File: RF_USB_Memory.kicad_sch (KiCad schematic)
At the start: 9 parts, among them J3 USB_B_Micro, U1 USBLC6-2SC6, U5 W25Q128JVSQ_SOIC208-mil

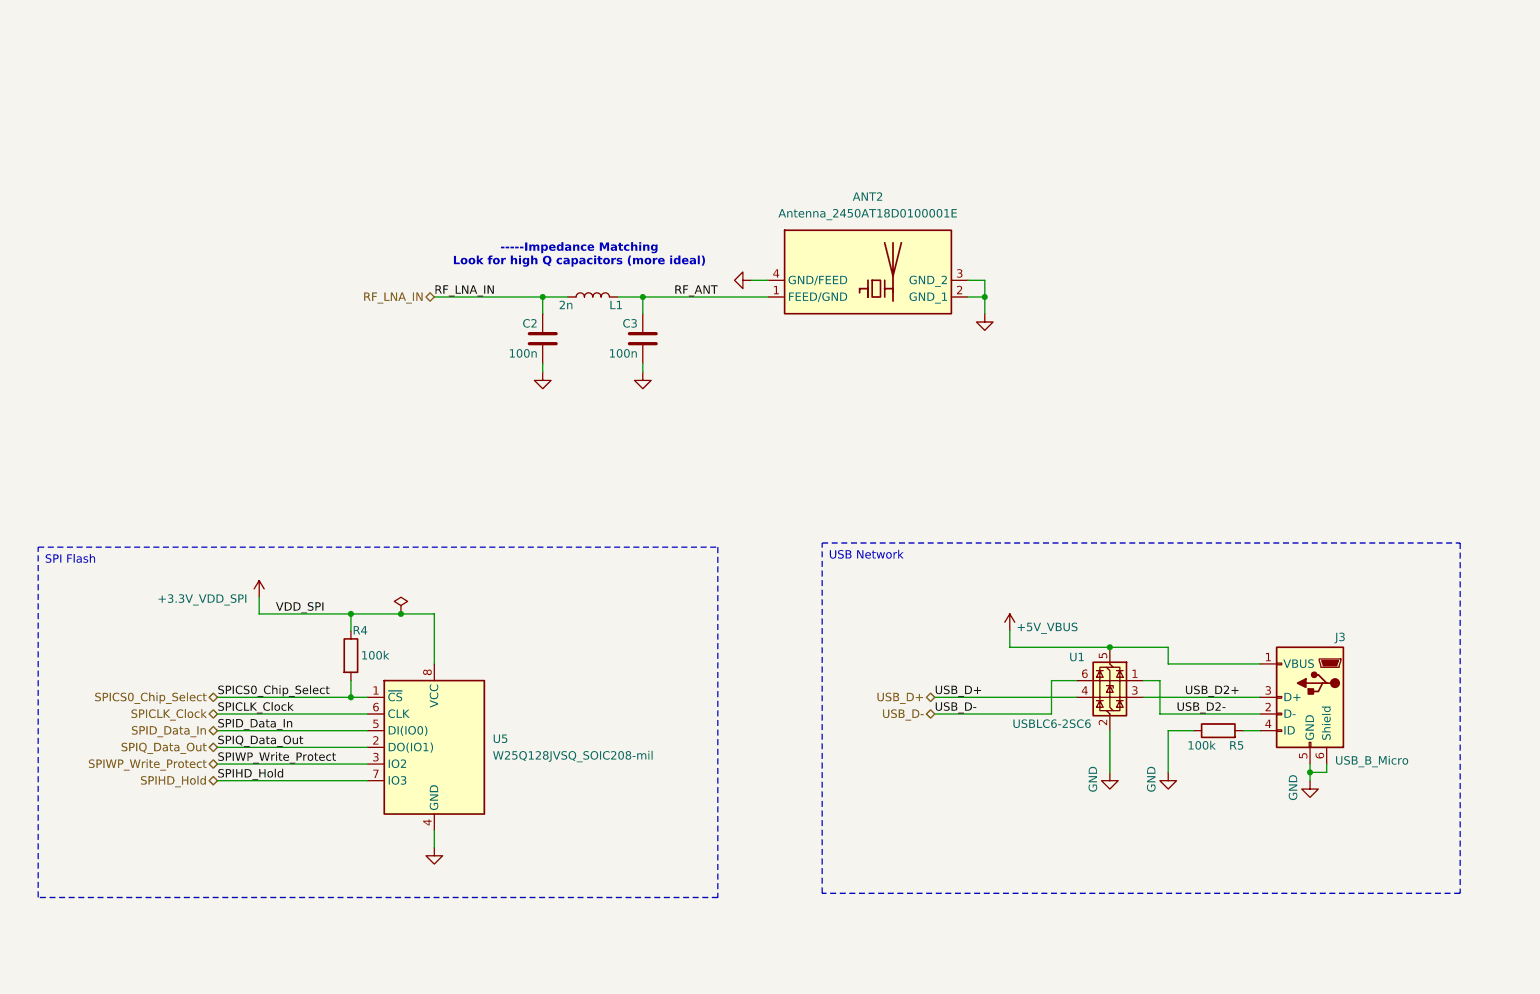
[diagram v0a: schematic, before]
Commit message: Update
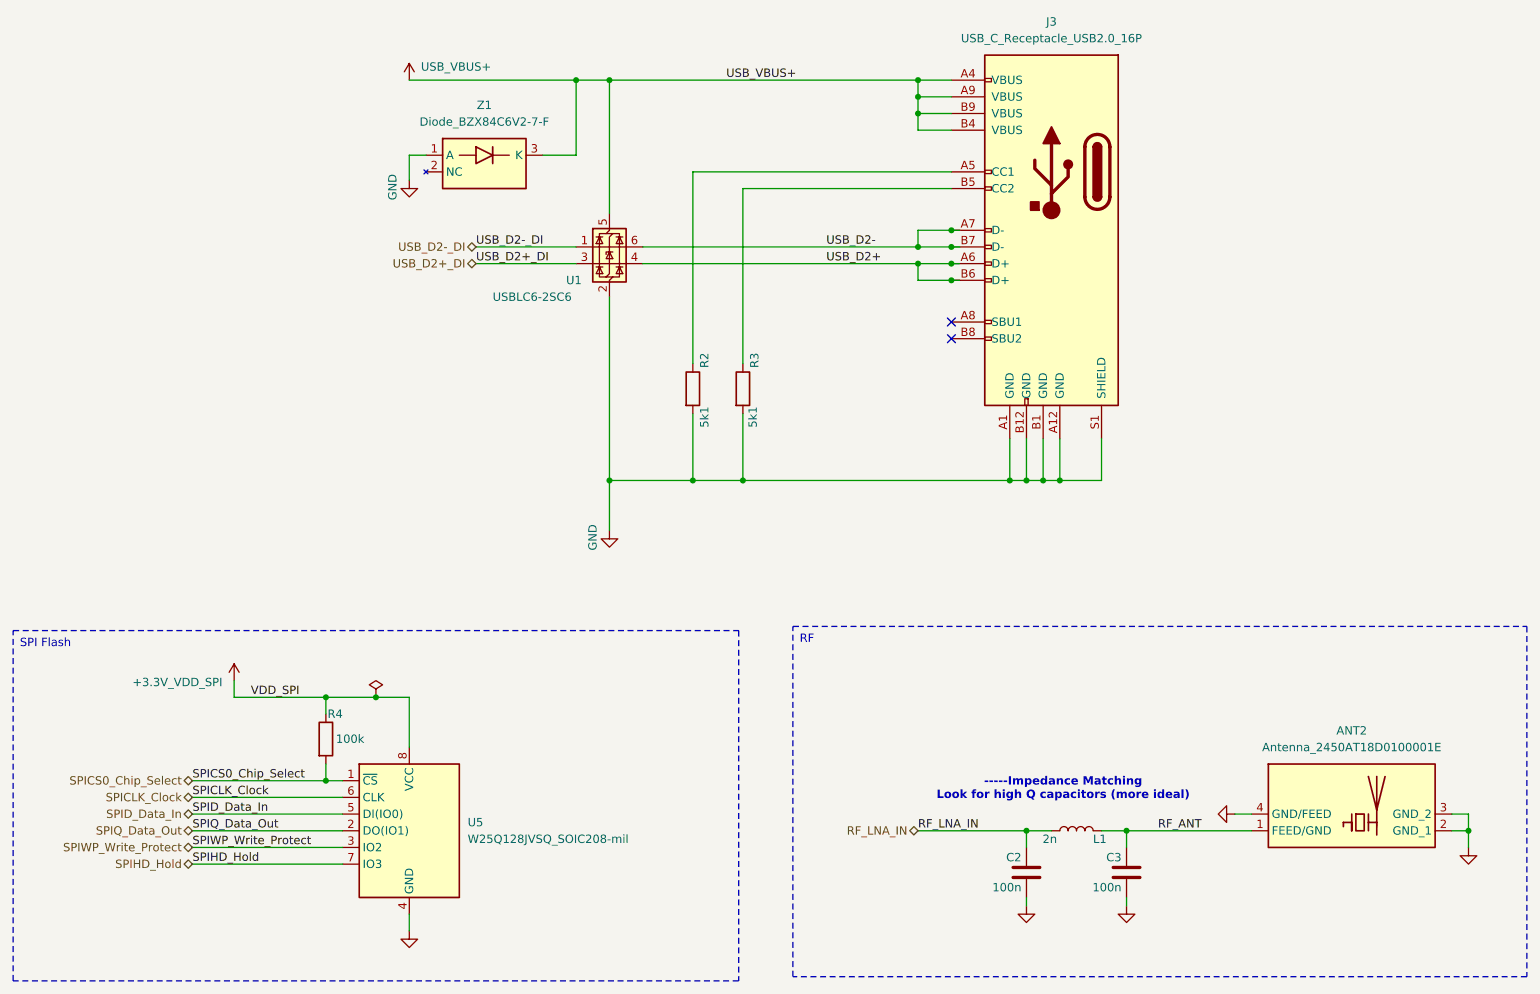
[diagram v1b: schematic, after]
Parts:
- removed J3: USB_B_Micro, Connector_USB:USB_Micro-B_Molex-105017-0001, symbol Connector:USB_B_Micro
- removed R5: 100k, Resistor_SMD:R_0805_2012Metric, symbol Device:R
- added J3: USB_C_Receptacle_USB2.0_16P, Connector_USB:USB_C_Receptacle_HRO_TYPE-C-31-M-12, symbol Connector:USB_C_Receptacle_USB2.0_16P
- added R2, R3: 5k1, Resistor_SMD:R_0805_2012Metric, symbol Device:R
- added Z1: Diode_BZX84C6V2-7-F, Personal_Project:Diode_BZX84C6V2_SOT96P240X110-3N, symbol Personal_Projects:Diode_BZX84C6V2-7-F
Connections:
- net USB_D+ is gone; now on net USB_D2+: U1.4 (I/O2)
- net USB_D- is gone; now on net USB_D2-: U1.6 (I/O1)
- net GND: now also J3.A1 (GND), J3.A12 (GND), J3.B1 (GND), J3.B12 (GND), J3.S1 (SHIELD), R2.2, R3.2, Z1.1 (A)
- net USB_D2+: now also J3.A6 (D+), J3.B6 (D+); no longer U1.3 (I/O2)
- net USB_D2-: now also J3.A7 (D-), J3.B7 (D-); no longer U1.1 (I/O1)
- net +5V_VBUS renamed USB_VBUS+
- net USB_VBUS+: now also J3.A4 (VBUS), J3.A9 (VBUS), J3.B4 (VBUS), J3.B9 (VBUS), Z1.3 (K)
- new net: J3.A5 (CC1), R2.1
- new net: J3.B5 (CC2), R3.1
- new net USB_D2+_DI: U1.3 (I/O2)
- new net USB_D2-_DI: U1.1 (I/O1)
- no-connect marks 0 -> 2
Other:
- moved on the sheet: ANT2, C2, C3, L1, R4, U5

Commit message: Update
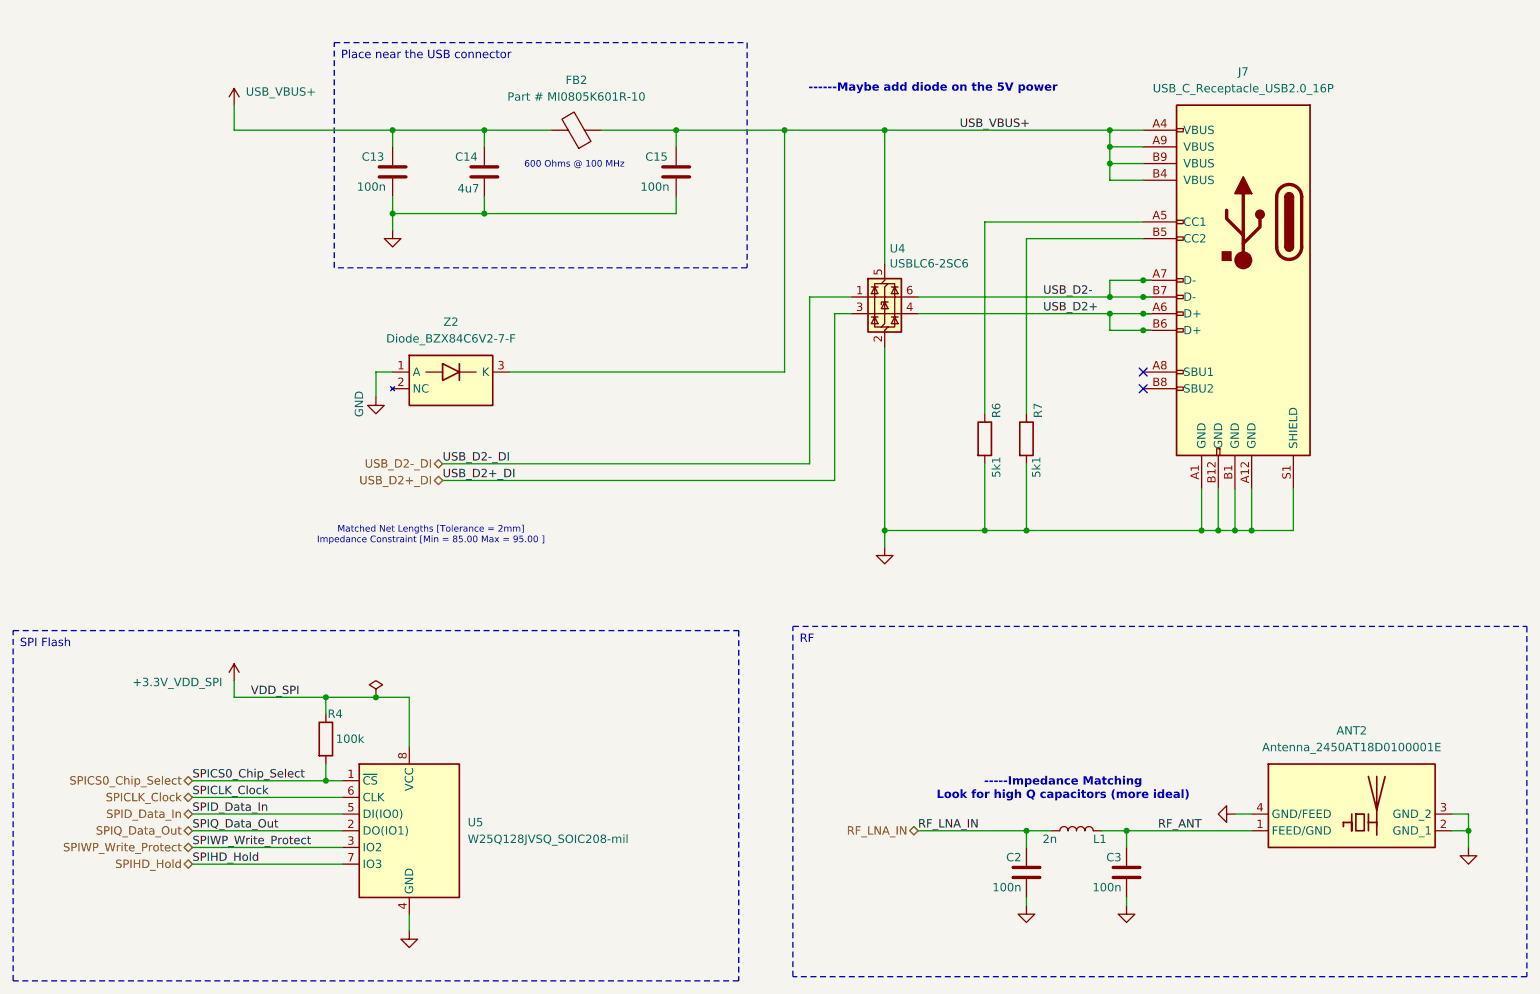
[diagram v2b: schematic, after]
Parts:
- removed J3: USB_C_Receptacle_USB2.0_16P, Connector_USB:USB_C_Receptacle_HRO_TYPE-C-31-M-12, symbol Connector:USB_C_Receptacle_USB2.0_16P
- removed R2, R3: 5k1, Resistor_SMD:R_0805_2012Metric, symbol Device:R
- removed U1: USBLC6-2SC6, Package_TO_SOT_SMD:SOT-23-6, symbol Power_Protection:USBLC6-2SC6
- removed Z1: Diode_BZX84C6V2-7-F, Personal_Project:Diode_BZX84C6V2_SOT96P240X110-3N, symbol Personal_Projects:Diode_BZX84C6V2-7-F
- added C13, C15: 100n, Capacitor_SMD:C_0805_2012Metric, symbol Device:C
- added C14: 4u7, Capacitor_SMD:C_0805_2012Metric, symbol Device:C
- added FB2: Part # MI0805K601R-10, Capacitor_SMD:C_0805_2012Metric, symbol Device:FerriteBead
- added J7: USB_C_Receptacle_USB2.0_16P, Connector_USB:USB_C_Receptacle_HRO_TYPE-C-31-M-12, symbol Connector:USB_C_Receptacle_USB2.0_16P
- added R6, R7: 5k1, Resistor_SMD:R_0805_2012Metric, symbol Device:R
- added U4: USBLC6-2SC6, Package_TO_SOT_SMD:SOT-23-6, symbol Power_Protection:USBLC6-2SC6
- added Z2: Diode_BZX84C6V2-7-F, Personal_Project:Diode_BZX84C6V2_SOT96P240X110-3N, symbol Personal_Projects:Diode_BZX84C6V2-7-F
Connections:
- net GND: now also C13.2, C14.2, C15.2, J7.A1 (GND), J7.A12 (GND), J7.B1 (GND), J7.B12 (GND), J7.S1 (SHIELD), R6.2, R7.2, U4.2 (GND), Z2.1 (A)
- net USB_D2+: now also J7.A6 (D+), J7.B6 (D+), U4.4 (I/O2)
- net USB_D2+_DI: now also U4.3 (I/O2)
- net USB_D2-: now also J7.A7 (D-), J7.B7 (D-), U4.6 (I/O1)
- net USB_D2-_DI: now also U4.1 (I/O1)
- net USB_VBUS+: now also C13.1, C14.1, C15.1, FB2.1, FB2.2, J7.A4 (VBUS), J7.A9 (VBUS), J7.B4 (VBUS), J7.B9 (VBUS), U4.5 (VBUS), Z2.3 (K)
- new net: J7.B5 (CC2), R7.1
- new net: J7.A5 (CC1), R6.1
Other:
- note added: "------Maybe add diode on the 5V power"
- note added: "600 Ohms @ 100 MHz"
- note added: "Matched Net Lengths [Tolerance = 2mm] Impedance Constraint [Min = 85.00 Max = 95.00 ]"
